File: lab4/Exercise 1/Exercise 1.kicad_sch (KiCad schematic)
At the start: 6 parts, among them SW1 SW_SPDT

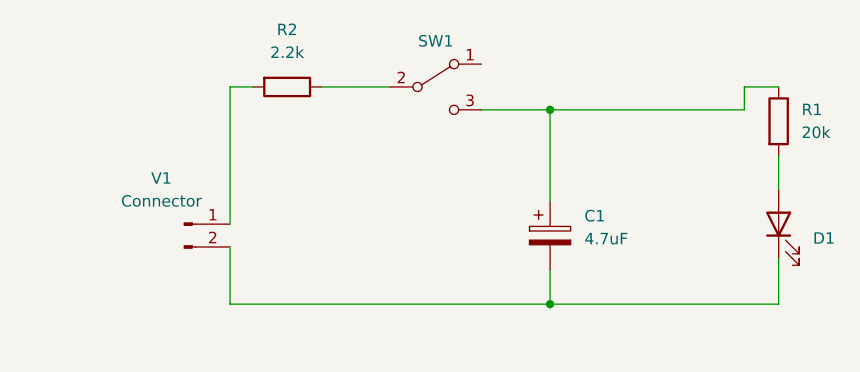
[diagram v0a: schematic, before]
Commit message: PCB Design
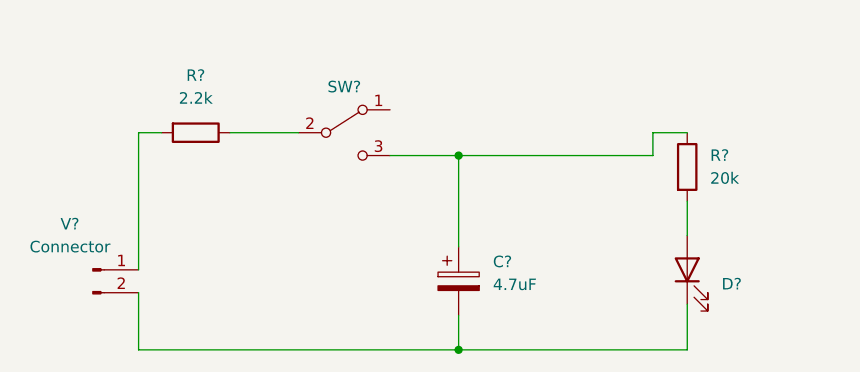
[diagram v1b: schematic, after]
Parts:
- removed C1: 4.7uF, symbol Device:C_Polarized
- removed D1: LED, symbol Device:LED
- removed R1: 20k, symbol Device:R
- removed R2: 2.2k, symbol Device:R
- removed SW1: SW_SPDT, symbol Switch:SW_SPDT
- removed V1: Connector, symbol Connector:Conn_01x02_Male
- added C?: 4.7uF, Capacitor_THT:C_Radial_D5.0mm_H5.0mm_P2.00mm, symbol Device:C_Polarized
- added D?: LED, LED_THT:LED_D5.0mm, symbol Device:LED
- added R?: 2.2k, Resistor_THT:R_Axial_DIN0516_L15.5mm_D5.0mm_P20.32mm_Horizontal, symbol Device:R
- added R?: 20k, Resistor_THT:R_Axial_DIN0516_L15.5mm_D5.0mm_P20.32mm_Horizontal, symbol Device:R
- added SW?: SW_SPDT, Button_Switch_THT:SW_E-Switch_EG1224_SPDT_Angled, symbol Switch:SW_SPDT
- added V?: Connector, Connector_JST:JST_PH_B2B-PH-K_1x02_P2.00mm_Vertical, symbol Connector:Conn_01x02_Male
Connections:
- new net: C?.1, R?.1, SW?.3 (C)
- new net: C?.2, D?.1 (K), V?.2 (Pin_2)
- new net: R?.2, V?.1 (Pin_1)
- new net: R?.1, SW?.2 (B)
- new net: D?.2 (A), R?.2
